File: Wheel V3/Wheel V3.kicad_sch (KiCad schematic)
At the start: 56 parts, among them J1 Motor_Off, J10 Conn_01x05, J11 Shift Register, J12 MT6835, J2 USB_C_Receptacle_USB2.0_16P, J3 Conn_01x07, J4 PWM_OUT, J5 CAN_Connector, J6 I2C_Connector, J7 E-Stop, J8 UART_Connector, J9 TEMP, SW1 SW_Push, SW2 SW_Push, U1 USBLC6-2SC6, U2 LDL111733R-3.3, U3 STM32F407VGTx, Y1 8MHz

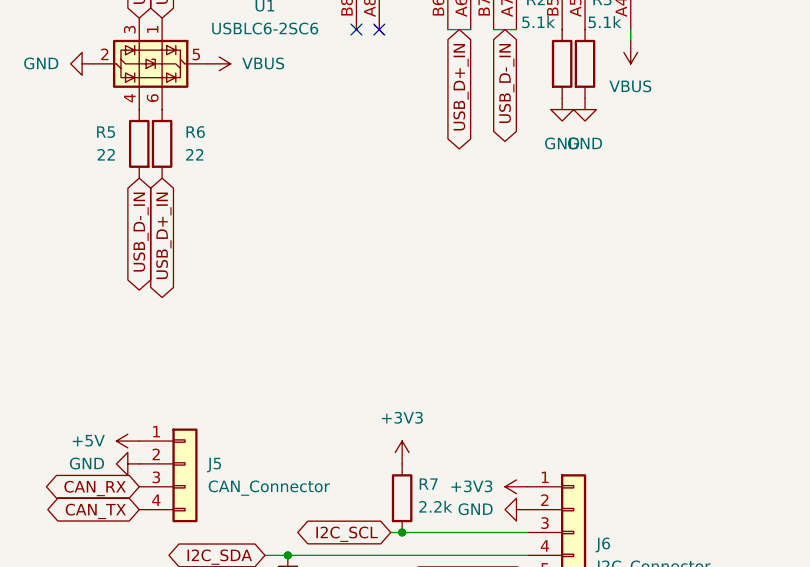
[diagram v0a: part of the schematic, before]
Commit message: Update
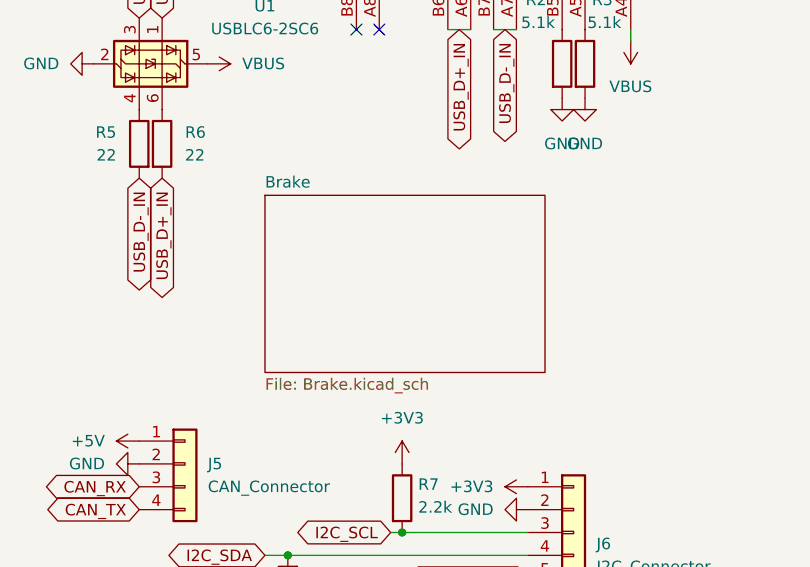
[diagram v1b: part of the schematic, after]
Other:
- added sheet Brake (Brake.kicad_sch)
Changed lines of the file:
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@@
+	)
+	(sheet
+		(at 238.76 57.785)
+		(size 31.115 19.685)
+		(exclude_from_sim no)
+		(in_bom yes)
+		(on_board yes)
+		(dnp no)
+		(fields_autoplaced yes)
+		(stroke
+			(width 0.1524)
+			(type solid)
+		)
+		(fill
+			(color 0 0 0 0)
+		)
+		(property "Sheetname" "Brake"
+			(at 238.76 57.0734 0)
+			(show_name no)
+			(do_not_autoplace no)
+			(effects
+				(font
+					(size 1.27 1.27)
+				)
+				(justify left bottom)
+			)
+		)
+		(property "Sheetfile" "Brake.kicad_sch"
+			(at 238.76 78.0546 0)
+			(show_name no)
+			(do_not_autoplace no)
+			(effects
+				(font
+					(size 1.27 1.27)
+				)
+				(justify left top)
+			)
+		)
+		(instances
+			(project "Wheel V3"
+				(path "/9ec62b0c-f2ce-42d9-a60a-bf785e542e97"
+					(page "3")
+				)
+			)
+		)
 	)
 	(sheet

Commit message: Update
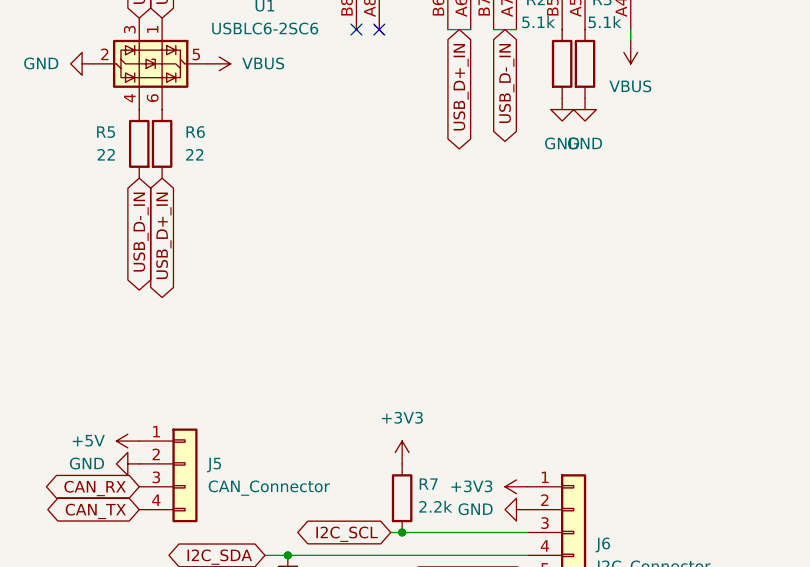
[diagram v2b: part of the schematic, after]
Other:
- removed sheet Brake
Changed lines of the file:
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@@
-	)
-	(sheet
-		(at 238.76 57.785)
-		(size 31.115 19.685)
-		(exclude_from_sim no)
-		(in_bom yes)
-		(on_board yes)
-		(dnp no)
-		(fields_autoplaced yes)
-		(stroke
-			(width 0.1524)
-			(type solid)
-		)
-		(fill
-			(color 0 0 0 0)
-		)
-		(property "Sheetname" "Brake"
-			(at 238.76 57.0734 0)
-			(show_name no)
-			(do_not_autoplace no)
-			(effects
-				(font
-					(size 1.27 1.27)
-				)
-				(justify left bottom)
-			)
-		)
-		(property "Sheetfile" "Brake.kicad_sch"
-			(at 238.76 78.0546 0)
-			(show_name no)
-			(do_not_autoplace no)
-			(effects
-				(font
-					(size 1.27 1.27)
-				)
-				(justify left top)
-			)
-		)
-		(instances
-			(project "Wheel V3"
-				(path "/9ec62b0c-f2ce-42d9-a60a-bf785e542e97"
-					(page "3")
-				)
-			)
-		)
 	)
 	(sheet
